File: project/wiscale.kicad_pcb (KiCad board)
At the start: 2 copper layers, 100 x 50 mm, 108 parts, among them J401 cell, J501 cell, J601 cell, J701 DS18B20, J801 DS18B20, J901 i2c, Q301 AO3401A, Q302 AO3401A, Q401 AO3401A, Q501 AO3401A, Q601 AO3401A, SW301 SW_SPDT, SW302 btn, U201 ESP-7(S) or ESP-12*, U301 BMS_USB_LiPo_Charger, U302 TPL5110, U401 HX711, U501 HX711, U601 HX711, U701 DS18B20Z, U702 DS18B20, U801 DS18B20Z, U802 DS18B20

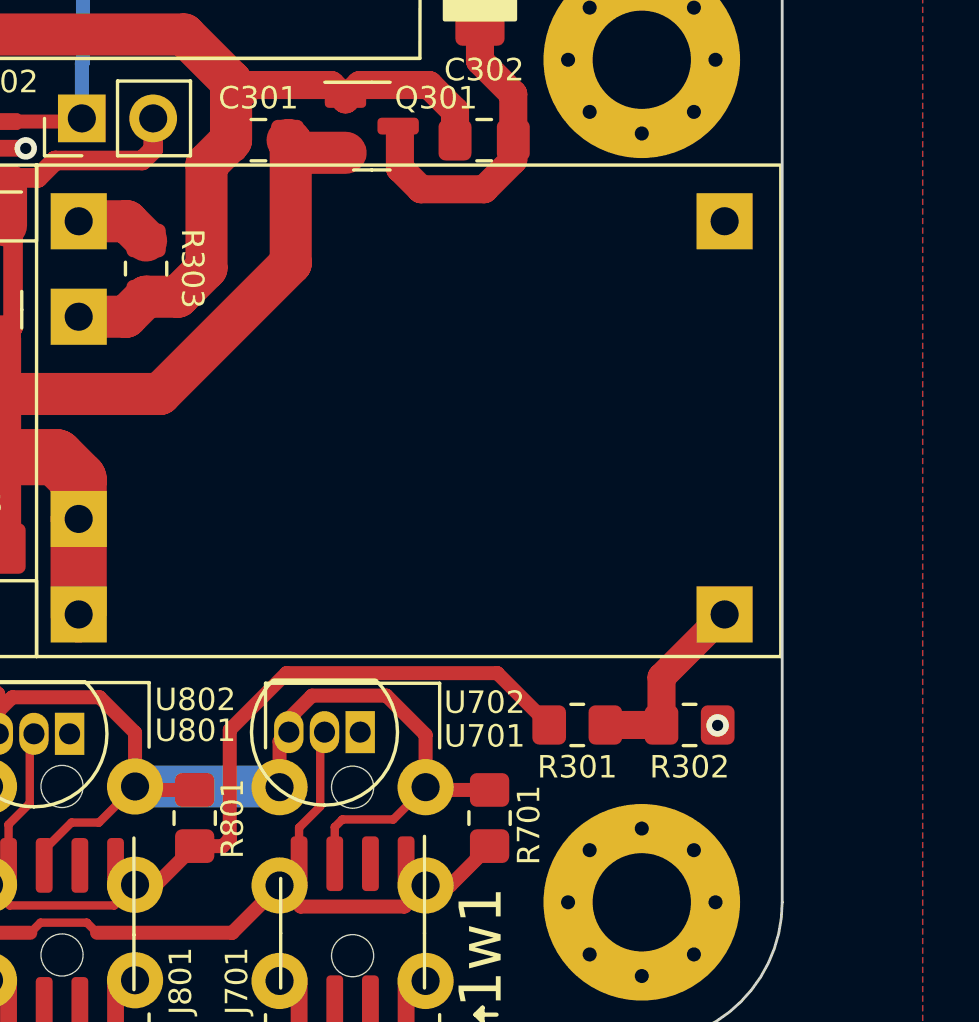
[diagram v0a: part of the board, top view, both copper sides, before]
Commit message: adding usb port with ldo and diode options
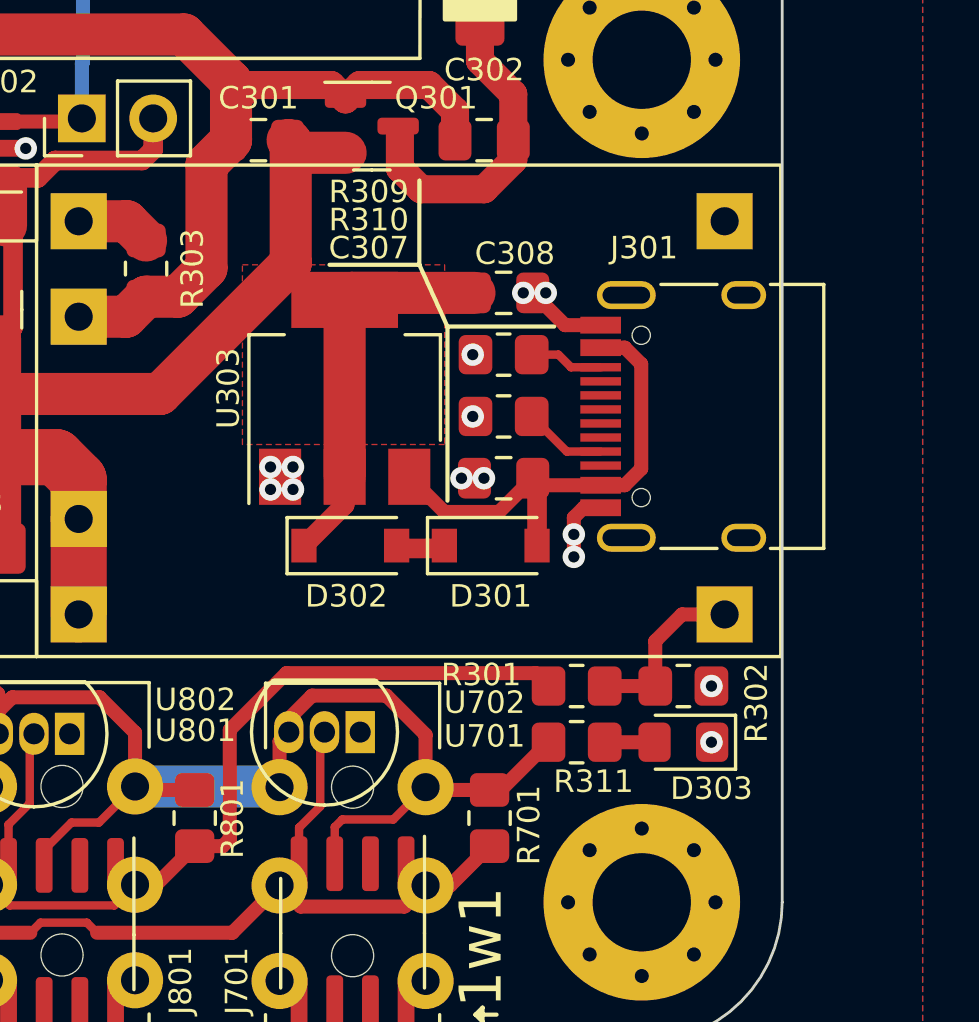
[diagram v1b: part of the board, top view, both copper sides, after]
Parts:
- added C307: 10u, Capacitor_SMD:C_0805_2012Metric_Pad1.18x1.45mm_HandSolder, F.Cu at (190.0, 95.4)
- added C308: 10u, Capacitor_SMD:C_0805_2012Metric_Pad1.18x1.45mm_HandSolder, F.Cu at (190.0, 88.8)
- added D301: 1N4148WL, Diode_SMD:D_SOD-123, F.Cu at (189.5, 97.8)
- added D302: 1N4148WL, Diode_SMD:D_SOD-123, F.Cu at (184.5, 97.8)
- added D303: GREEN, LED_SMD:LED_0805_2012Metric_Pad1.15x1.40mm_HandSolder, F.Cu at (196.4, 104.8)
- added J301: USB_POWER_IN, -local:USB_C_Receptacle_HRO_TYPE-C-31-M-12, F.Cu at (197.5, 93.2)
- added R309: 4k7, Resistor_SMD:R_0805_2012Metric_Pad1.20x1.40mm_HandSolder, F.Cu at (190.0, 91.0)
- added R310: 4k7, Resistor_SMD:R_0805_2012Metric_Pad1.20x1.40mm_HandSolder, F.Cu at (190.0, 93.2)
- added R311: 4k7, Resistor_SMD:R_0805_2012Metric_Pad1.20x1.40mm_HandSolder, F.Cu at (192.6, 104.8)
- added U303: AMS1117-3.3, Package_TO_SOT_SMD:SOT-223-3_TabPin2, F.Cu at (184.3, 92.2)
- moved G*** 56.0 mm to (132.5, 77.5)
- moved R302 1.40 mm to (196.4, 102.8)
- moved R301 1.39 mm to (192.6, 102.8)
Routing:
- net /PSU/_usb_vbus: track 0.00 -> 17.5 mm
- net Vbat: track 49.8 -> 63.9 mm
- net GND: track 62.9 -> 68.3 mm, vias 168 -> 181
- net /PSU/_cc1: track 0.00 -> 2.97 mm
- net /ADC1/Vcc: track 190.6 -> 193.4 mm
- net /PSU/_cc2: track 0.00 -> 2.64 mm
- net Net-(D303-Pad2): track 0.00 -> 1.78 mm
- net Net-(D301-Pad1): track 0.00 -> 1.74 mm
- net /PSU/_vusb: track 6.87 -> 6.26 mm
- net /MCU/Charging: track 99.4 -> 98.8 mm
- added copper zone on F.Cu, net Vbat
